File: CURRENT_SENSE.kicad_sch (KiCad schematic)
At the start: 11 parts, among them U4 3PEAK TP09-SR

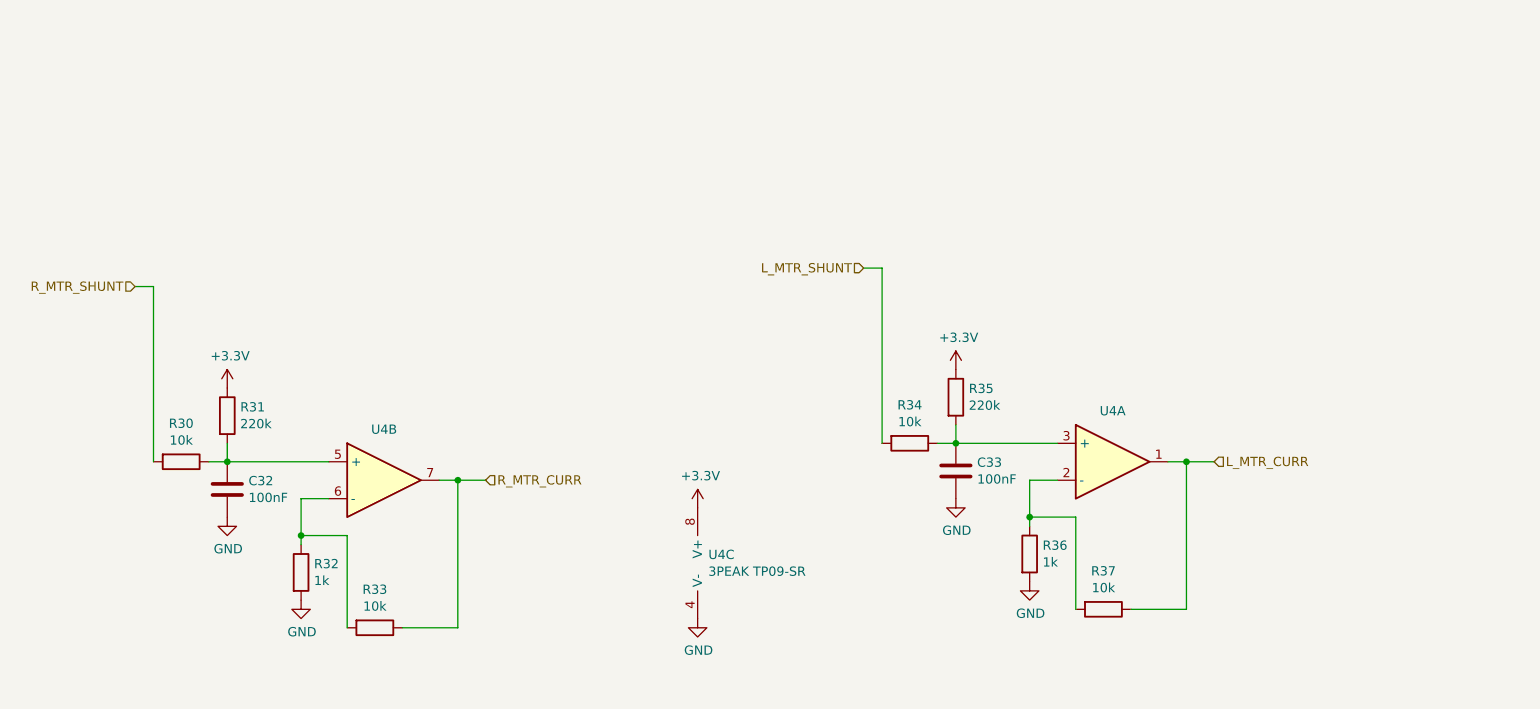
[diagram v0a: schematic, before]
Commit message: Updated Current sense circuit
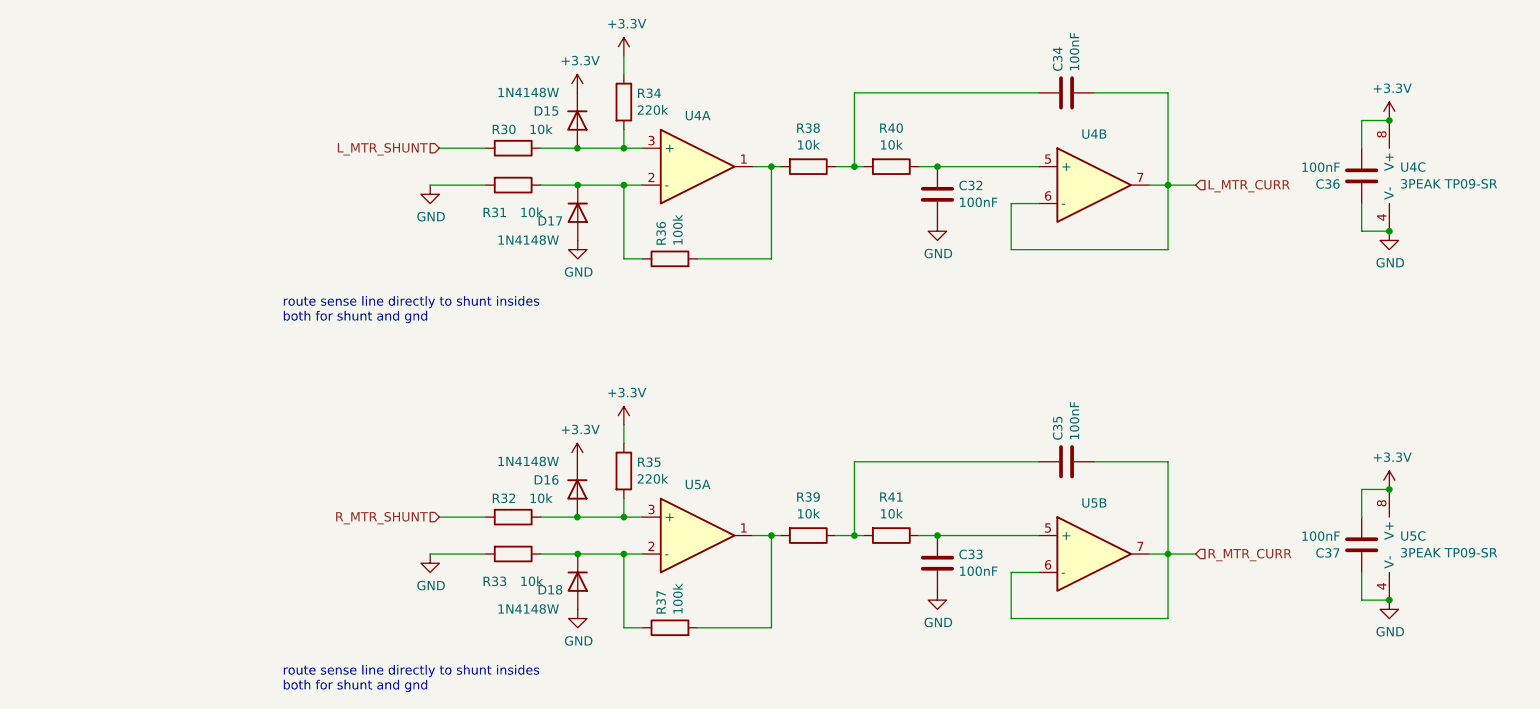
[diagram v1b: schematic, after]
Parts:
- removed C33: 100nF, Capacitor_SMD:C_0603_1608Metric, symbol Device:C
- removed R35: 220k, Resistor_SMD:R_0603_1608Metric, symbol Device:R
- added C32, C34, C35, C36, C37: 100nF, Capacitor_SMD:C_0603_1608Metric, symbol Device:C
- added D15, D16, D17, D18: 1N4148W, Diode_SMD:D_SOD-123, symbol Device:D
- added R30, R31, R38, R39, R40: 10k, Resistor_SMD:R_0603_1608Metric, symbol Device:R
- added U4: 3PEAK TP09-SR, Package_SO:SOIC-8_3.9x4.9mm_P1.27mm, symbol Device:Opamp_Dual_Generic
- R32: value 1k -> 10k; LCSC Part # C21190 -> C25804
- R34: value 10k -> 220k; LCSC Part # C25804 -> C22961
- R36: value 1k -> 100k; LCSC Part # C21190 -> (none)
- R37: value 10k -> 100k; LCSC Part # C25804 -> (none)
- renumbered C32 to C33, R31 to R35, R30 to R41, U4 to U5
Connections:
- net +3V3: now also R34.1, C36.2, C37.2, D15.1 (K), D16.1 (K), U4.8 (V+)
- net GND: now also R33.2, C32.2, C36.1, C37.1, D17.2 (A), D18.2 (A), R31.2, U4.4 (V-); no longer R32.2, R36.2
- net L_MTR_CURR: now also C34.2, U4.6 (-), U4.7; no longer R37.1, U5.1
- net L_MTR_SHUNT: now also R30.2; no longer R34.2
- net R_MTR_CURR: now also U5.6 (-), C35.2; no longer R33.1
- net R_MTR_SHUNT: now also R32.2; no longer R41.2
- net at C33.1, R41.1, U5.5 (+): no longer R35.2
- net at U5.3 (+): now also R32.1, R35.2, D16.2 (A); no longer R34.1
- new net: C35.1, R39.1, R41.2
- new net: D18.1 (K), R33.1, R37.1, U5.2 (-)
- new net: R37.2, R39.2, U5.1
- new net: D15.2 (A), R30.1, R34.2, U4.3 (+)
- new net: C32.1, R40.1, U4.5 (+)
- new net: C34.1, R38.1, R40.2
- new net: D17.1 (K), R31.1, R36.1, U4.2 (-)
- new net: R36.2, R38.2, U4.1
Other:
- note added: "route sense line directly to shunt insides both for shunt and gnd"
- moved on the sheet: C33, R33, R35, R41, U5A, U5B, U5C
